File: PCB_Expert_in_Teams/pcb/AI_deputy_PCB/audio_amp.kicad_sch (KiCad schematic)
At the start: 19 parts, among them IC4 IS31AP2005-SLS2-TR, IC5 IS31AP2005-SLS2-TR, J13 Conn_01x02_Socket, J14 Conn_01x02_Socket, J8 Conn_01x04_Socket

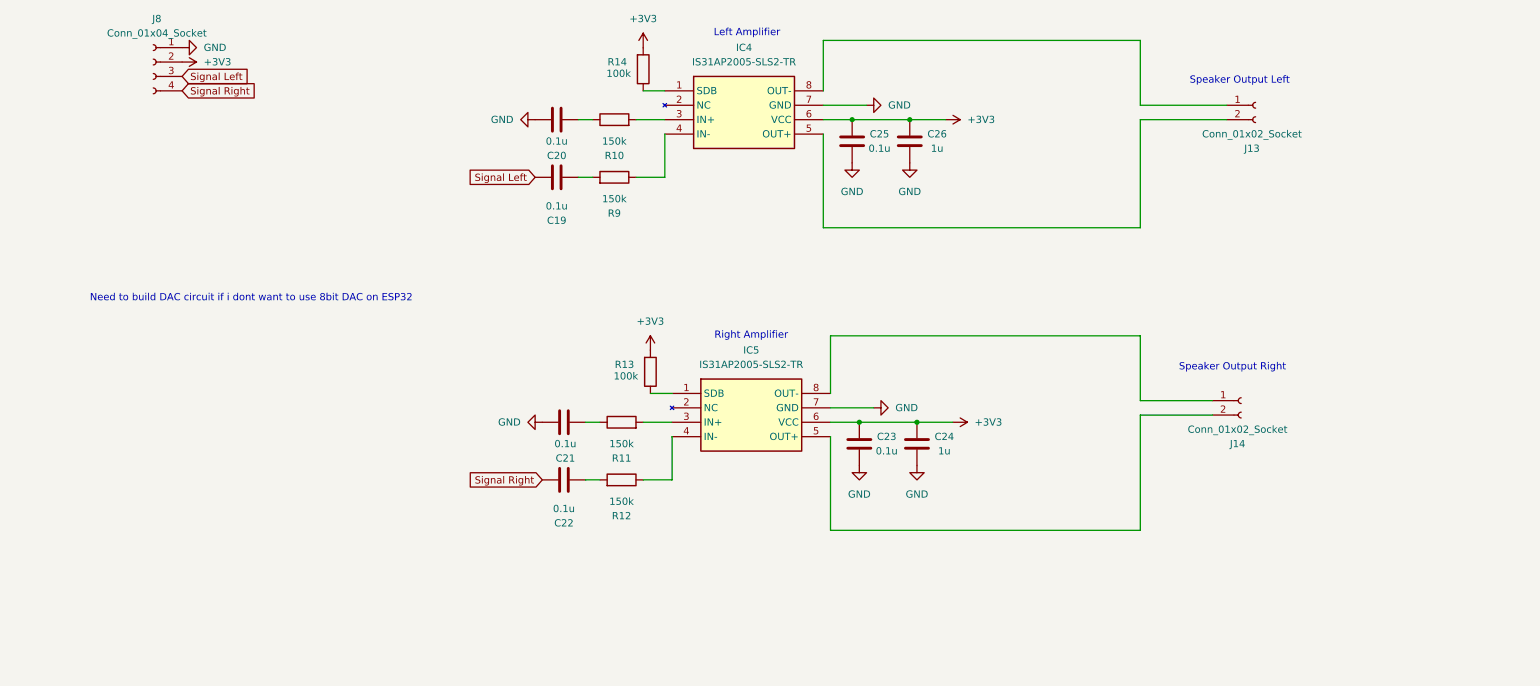
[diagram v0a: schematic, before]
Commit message: update schematic from desktop
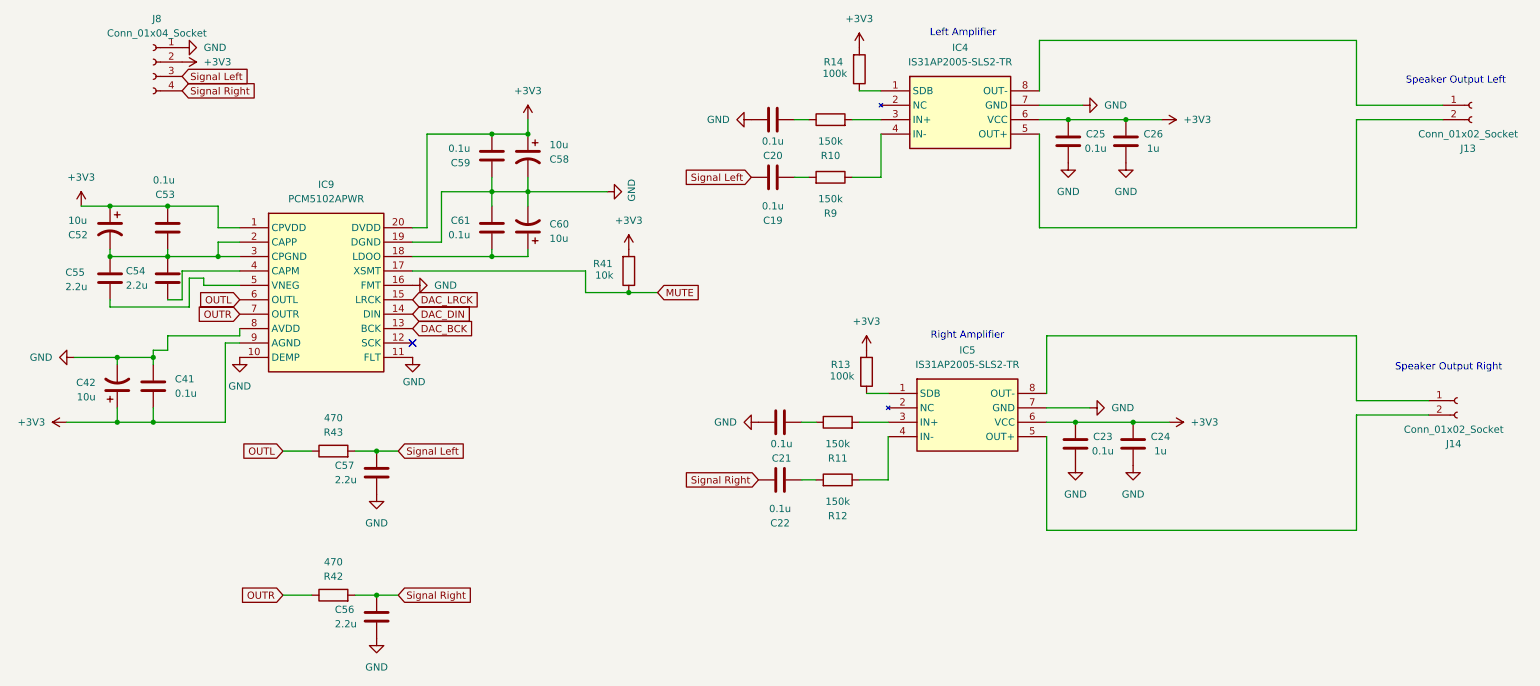
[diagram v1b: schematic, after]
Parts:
- added C41, C53, C59, C61: 0.1u, Capacitor_SMD:C_0805_2012Metric_Pad1.18x1.45mm_HandSolder, symbol Device:C
- added C42, C52, C58, C60: 10u, Capacitor_SMD:CP_Elec_4x5.4, symbol Device:C_Polarized_US
- added C54, C55, C56, C57: 2.2u, Capacitor_SMD:C_0805_2012Metric_Pad1.18x1.45mm_HandSolder, symbol Device:C
- added IC9: PCM5102APWR, SOP65P640X120-20N, symbol DAC-PCM510:PCM5102APWR
- added R41: 10k, Resistor_SMD:R_0805_2012Metric_Pad1.20x1.40mm_HandSolder, symbol Device:R
- added R42, R43: 470, Resistor_SMD:R_0805_2012Metric_Pad1.20x1.40mm_HandSolder, symbol Device:R
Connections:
- net +3V3: now also C41.2, C42.1, C52.1, C53.2, C58.1, C59.2, IC9.1 (CPVDD), IC9.20 (DVDD), IC9.9 (AGND), R41.2
- net GND: now also C41.1, C42.2, C56.2, C57.2, C58.2, C59.1, C60.2, C61.1, IC9.10 (DEMP), IC9.11 (FLT), IC9.16 (FMT), IC9.19 (DGND), IC9.8 (AVDD)
- net Signal Left: now also C57.1, R43.2
- net Signal Right: now also C56.1, R42.2
- new net: C52.2, C53.1, C54.1, C55.1, IC9.2 (CAPP), IC9.3 (CPGND)
- new net: C60.1, C61.2, IC9.18 (LDOO)
- new net: C54.2, IC9.4 (CAPM)
- new net: C55.2, IC9.5 (VNEG)
- new net DAC_BCK: IC9.13 (BCK)
- new net DAC_DIN: IC9.14 (DIN)
- new net DAC_LRCK: IC9.15 (LRCK)
- new net MUTE: IC9.17 (XSMT), R41.1
- new net OUTL: IC9.6 (OUTL), R43.1
- new net OUTR: IC9.7 (OUTR), R42.1
- no-connect marks 0 -> 1
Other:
- note removed: "Need to build DAC circuit if i dont want to use 8bit DAC on ESP32"
- moved on the sheet: C19, C20, C21, C22, C23, C24, C25, C26, IC4, IC5, J13, J14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
